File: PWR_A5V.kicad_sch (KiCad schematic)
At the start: 7 parts, among them Q4 STS5DNF60L

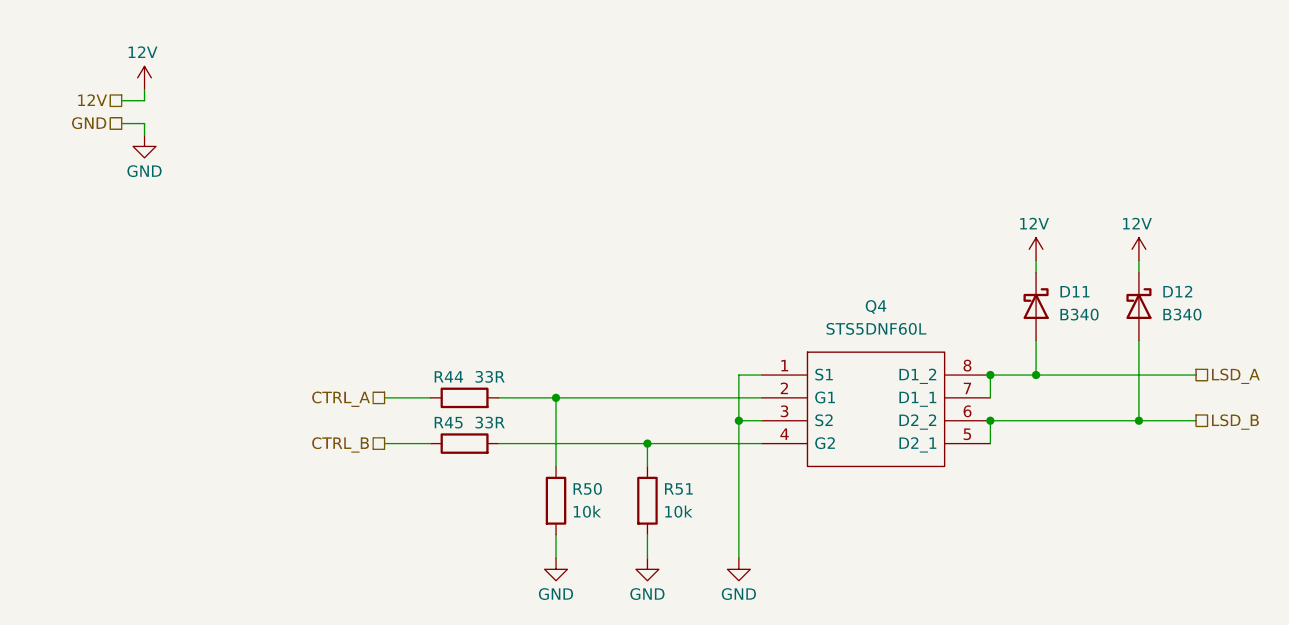
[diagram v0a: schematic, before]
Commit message: possible working power mux
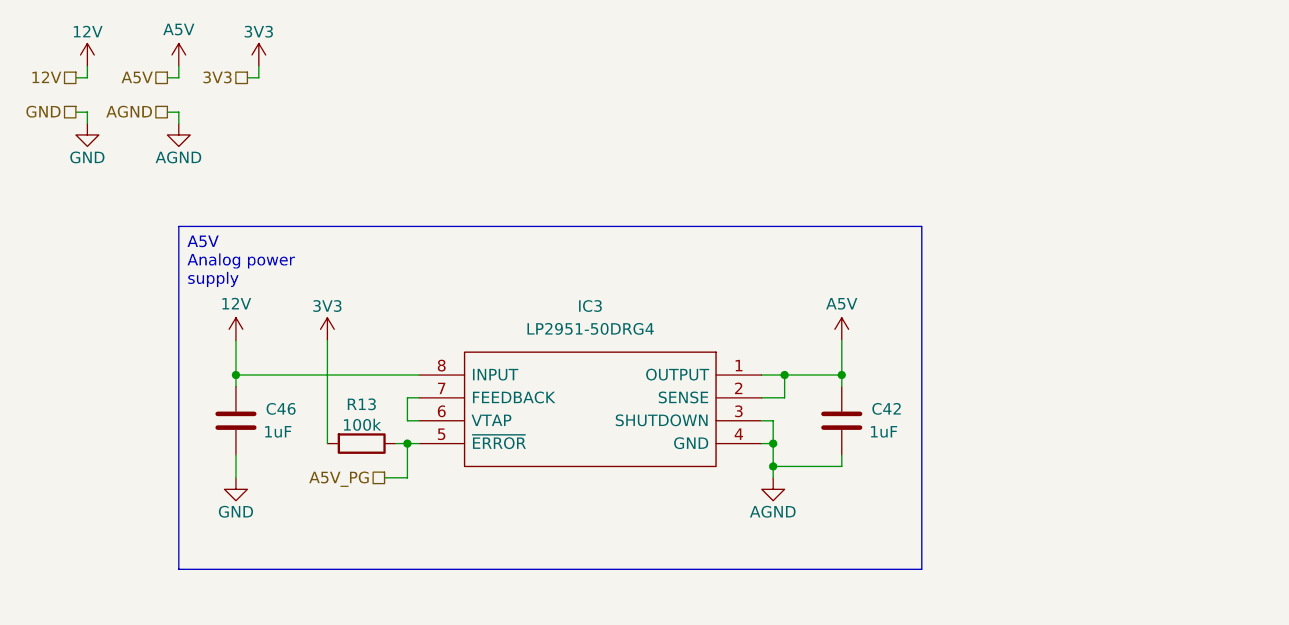
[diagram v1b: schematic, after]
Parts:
- removed D11, D12: B340, Diode_SMD:D_SMC, symbol Diode:B340
- removed Q4: STS5DNF60L, SOIC127P600X175-8N, symbol 0_SamacSys_Parts:STS5DNF60L
- removed R44, R45: 33R, Resistor_SMD:R_0603_1608Metric_Pad0.98x0.95mm_HandSolder, symbol Device:R
- removed R50, R51: 10k, symbol Device:R
- added C42, C46: 1uF, Capacitor_SMD:C_0603_1608Metric_Pad1.08x0.95mm_HandSolder, symbol Device:C
- added IC3: LP2951-50DRG4, SOIC127P600X175-8N, symbol 0_SamacSys_Parts:LP2951-50DRG4
- added R13: 100k, Resistor_SMD:R_0603_1608Metric_Pad0.98x0.95mm_HandSolder, symbol Device:R
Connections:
- net 12V: now also C46.1, IC3.8 (INPUT)
- net GND: now also C46.2
- new net: IC3.6 (VTAP), IC3.7 (FEEDBACK)
- new net 3V3: R13.2
- new net A5V: C42.1, IC3.1 (OUTPUT), IC3.2 (SENSE)
- new net A5V_PG: IC3.5 (~{ERROR}), R13.1
- new net AGND: C42.2, IC3.3 (SHUTDOWN), IC3.4 (GND)
